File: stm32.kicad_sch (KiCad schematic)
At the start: 62 parts, among them J401 Conn_02x07_Odd_Even, J402 Conn_01x02, J403 Conn_01x02, J404 Conn_01x07, J405 Conn_01x03, J406 Conn_01x07, J407 Conn_01x03, J408 Conn_01x05, J409 Conn_01x05, J410 Conn_01x04, J411 Conn_01x03, J412 Conn_01x07, SW401 SW_MEC_5E, SW402 SW_MEC_5E, U401 STM32G070RBT6, Y401 16 Mhz

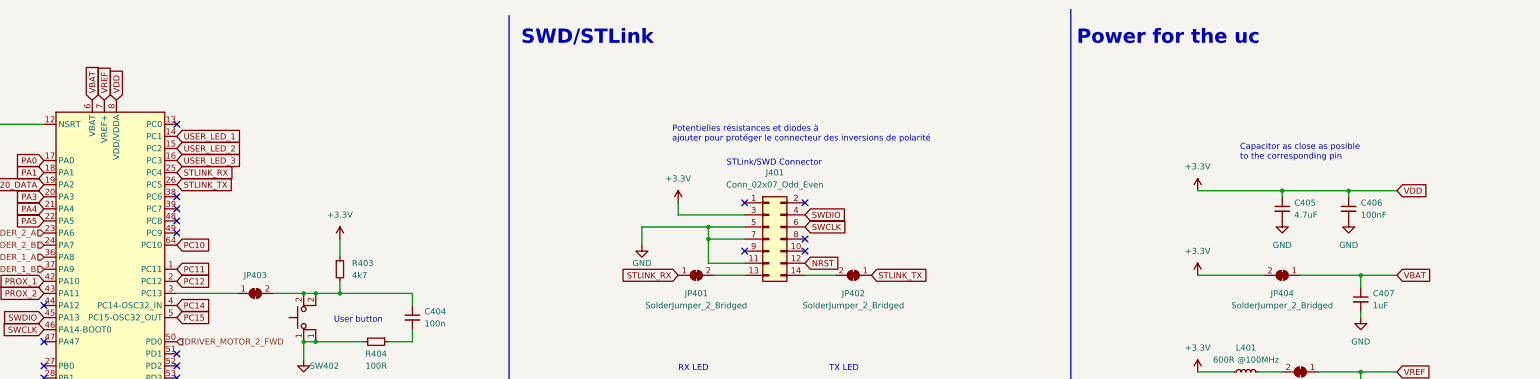
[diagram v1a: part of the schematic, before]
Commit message: Prof approved commit
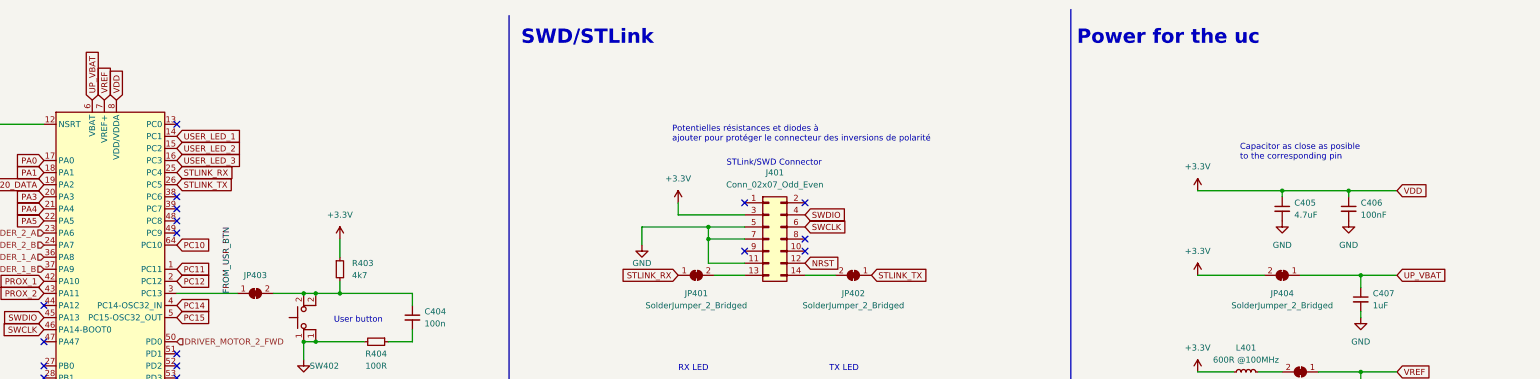
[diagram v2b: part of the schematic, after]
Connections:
- net FROM_USR_BTN: now reaches JP403.1 (A), U401.3 (PC13)
- net VBAT renamed UP_VBAT
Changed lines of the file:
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@@
     (effects (font (size 3 3) (thickness 0.6) bold) (justify left bottom))
+  )
+  (label "FROM_USR_BTN" (at 118.11 71.12 90)
+    (effects (font (size 1.27 1.27)) (justify left bottom))
   )
   (global_label "I2C1_SDL" (shape input) (at 78.74 106.68 180) (fields_autoplaced)
@@
     )
   )
-  (global_label "VBAT" (shape input) (at 363.22 67.31 0) (fields_autoplaced)
+  (global_label "UP_VBAT" (shape input) (at 363.22 67.31 0) (fields_autoplaced)
     (effects (font (size 1.27 1.27)) (justify left))
-    (property "Intersheet References" "${INTERSHEET_REFS}" (id 0) (at 370.0479 67.2306 0)
+    (property "Intersheet References" "${INTERSHEET_REFS}" (id 0) (at 373.616 67.2306 0)
       (effects (font (size 1.27 1.27)) (justify left) hide)
     )
@@
     )
   )
-  (global_label "VBAT" (shape input) (at 88.9 30.48 90) (fields_autoplaced)
+  (global_label "UP_VBAT" (shape input) (at 88.9 30.48 90) (fields_autoplaced)
     (effects (font (size 1.27 1.27)) (justify left))
-    (property "Références Inter-Feuilles" "${INTERSHEET_REFS}" (id 0) (at 88.8206 23.6521 90)
+    (property "Références Inter-Feuilles" "${INTERSHEET_REFS}" (id 0) (at 88.8206 20.084 90)
       (effects (font (size 1.27 1.27)) (justify left) hide)
     )
